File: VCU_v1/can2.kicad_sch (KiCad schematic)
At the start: 6 parts, among them U12 MCP2562FD-E/SN

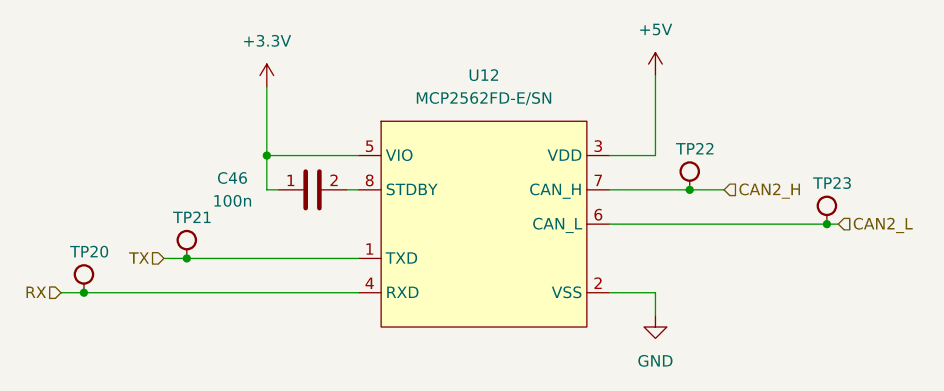
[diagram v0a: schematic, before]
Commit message: almost done i promise
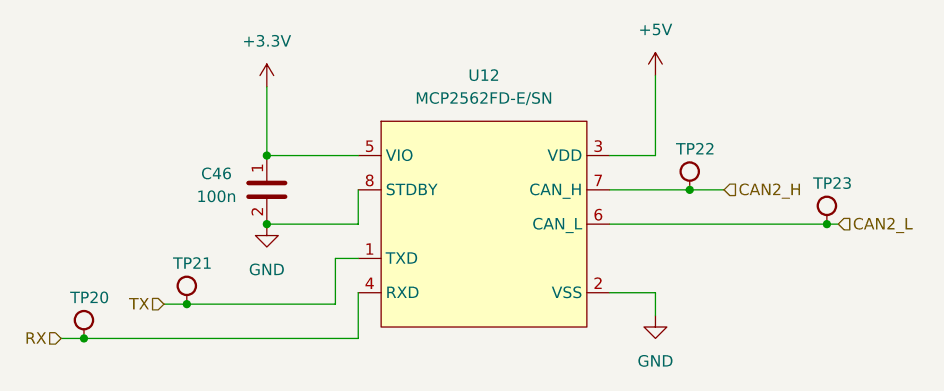
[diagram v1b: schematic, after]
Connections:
- net GND: now also C46.2, U12.8 (STDBY)
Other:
- moved on the sheet: C46, TP20, TP21
